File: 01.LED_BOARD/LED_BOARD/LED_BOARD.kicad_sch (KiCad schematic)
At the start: 4 parts, among them SW1 SW_DPDT_x2

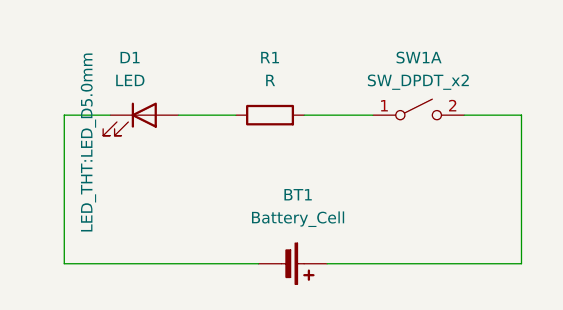
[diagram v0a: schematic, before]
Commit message: LED BOARD - EESCHEMA - COMMENT
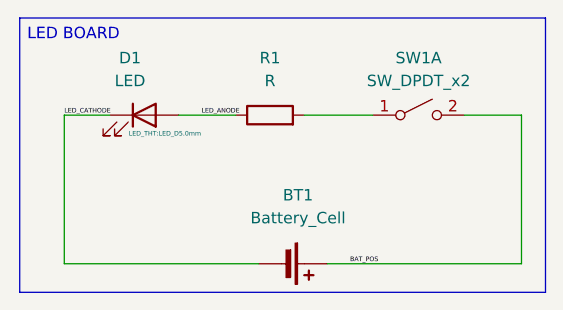
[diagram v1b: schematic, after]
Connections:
- net LED_CATHODE: now reaches BT1.2 (-), D1.1 (K)
- net LED_ANODE: now reaches D1.2 (A), R1.1
- net BAT_POS: now reaches BT1.1 (+), SW1.2 (B)
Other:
- note added: "LED BOARD"
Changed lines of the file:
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@@
 		(company "GOBAL KRISHNAN ")
+	)
+	(rectangle
+		(start 147.447 74.295)
+		(end 205.867 104.775)
+		(stroke
+			(width 0)
+			(type default)
+		)
+		(fill
+			(type none)
+		)
+	)
+	(text "LED BOARD\n"
+		(exclude_from_sim no)
+		(at 153.416 76.2 0)
+		(effects
+			(font
+				(size 1.27 1.27)
+			)
+		)
 	)
 	(wire
@@
 		)
 	)
+	(label "BAT_POS"
+		(at 184.15 101.6 0)
+		(effects
+			(font
+				(size 0.508 0.508)
+			)
+			(justify left bottom)
+		)
+	)
+	(label "LED_ANODE"
+		(at 167.64 85.09 0)
+		(effects
+			(font
+				(size 0.508 0.508)
+			)
+			(justify left bottom)
+		)
+	)
+	(label "LED_CATHODE"
+		(at 152.4 85.09 0)
+		(effects
+			(font
+				(size 0.508 0.508)
+			)
+			(justify left bottom)
+		)
+	)
 	(symbol
 		(lib_id "Device:LED")
@@
 		)
 		(property "Footprint" "LED_THT:LED_D5.0mm"
-			(at 154.94 88.138 90)
+			(at 163.576 87.122 0)
 			(effects
 				(font
-					(size 1.27 1.27)
+					(size 0.508 0.508)
 				)
 			)
